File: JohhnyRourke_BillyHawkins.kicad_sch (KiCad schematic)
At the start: 12 parts, among them J1 Power In, J2 Motor Out, U2 DRV8873HPWPRQ1

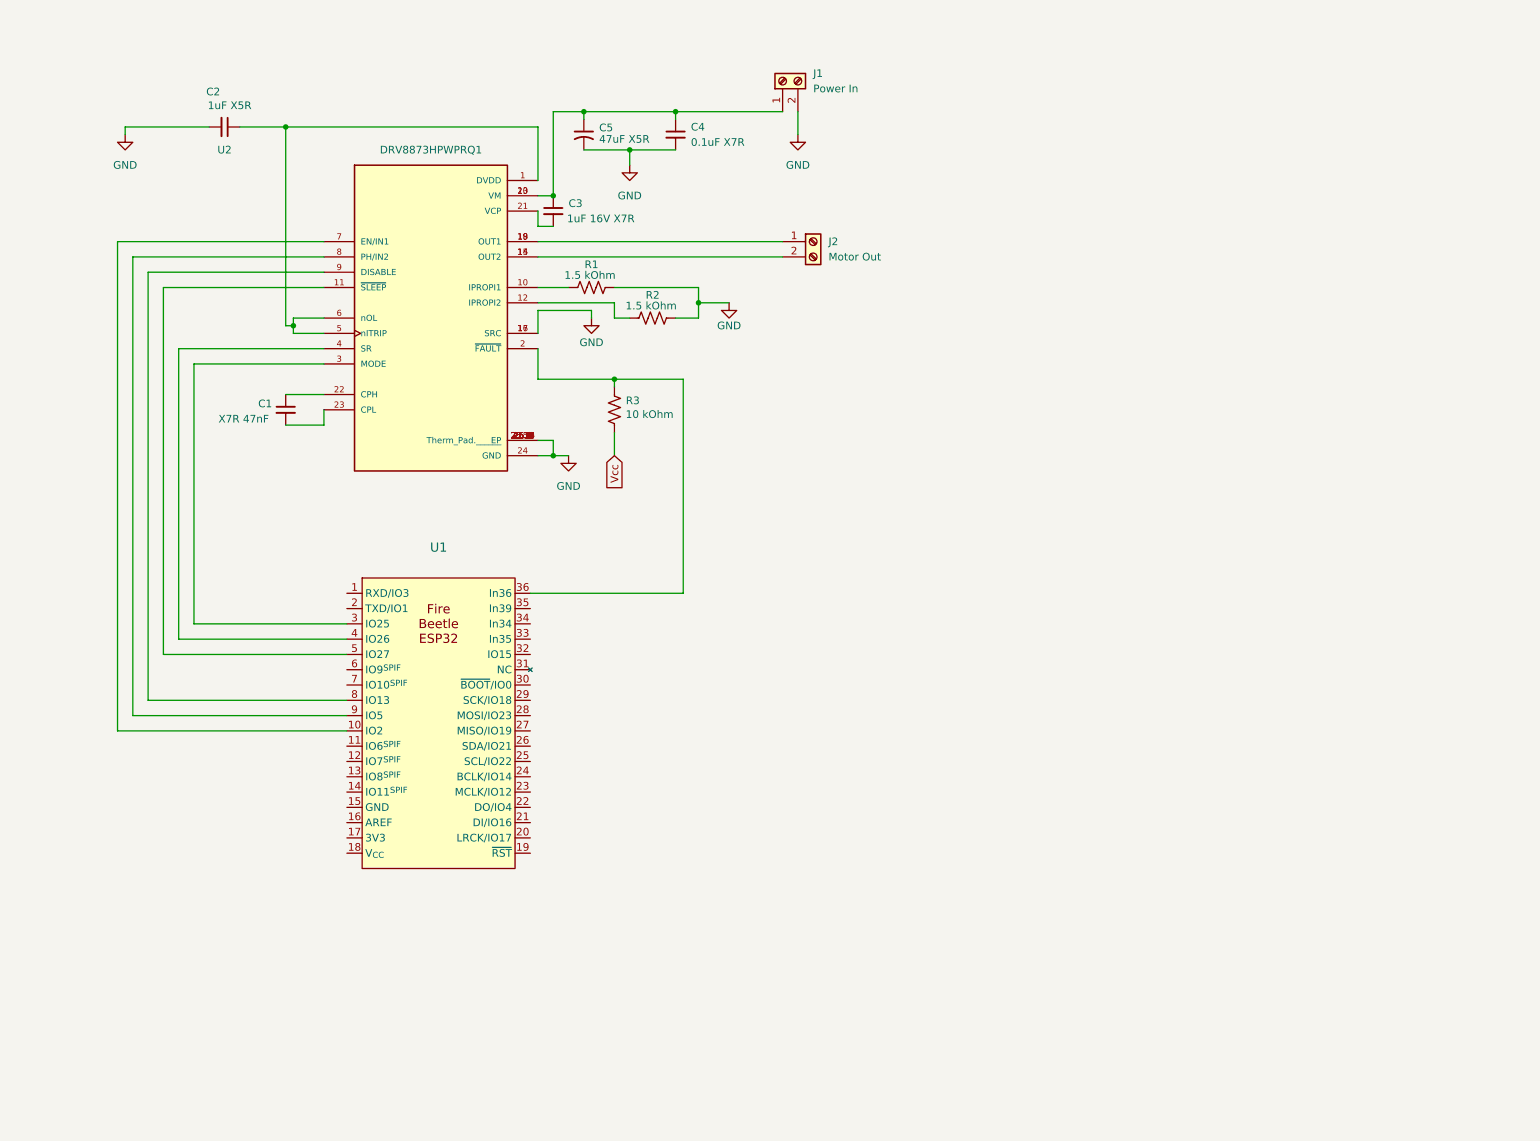
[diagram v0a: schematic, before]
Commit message: Add files via upload
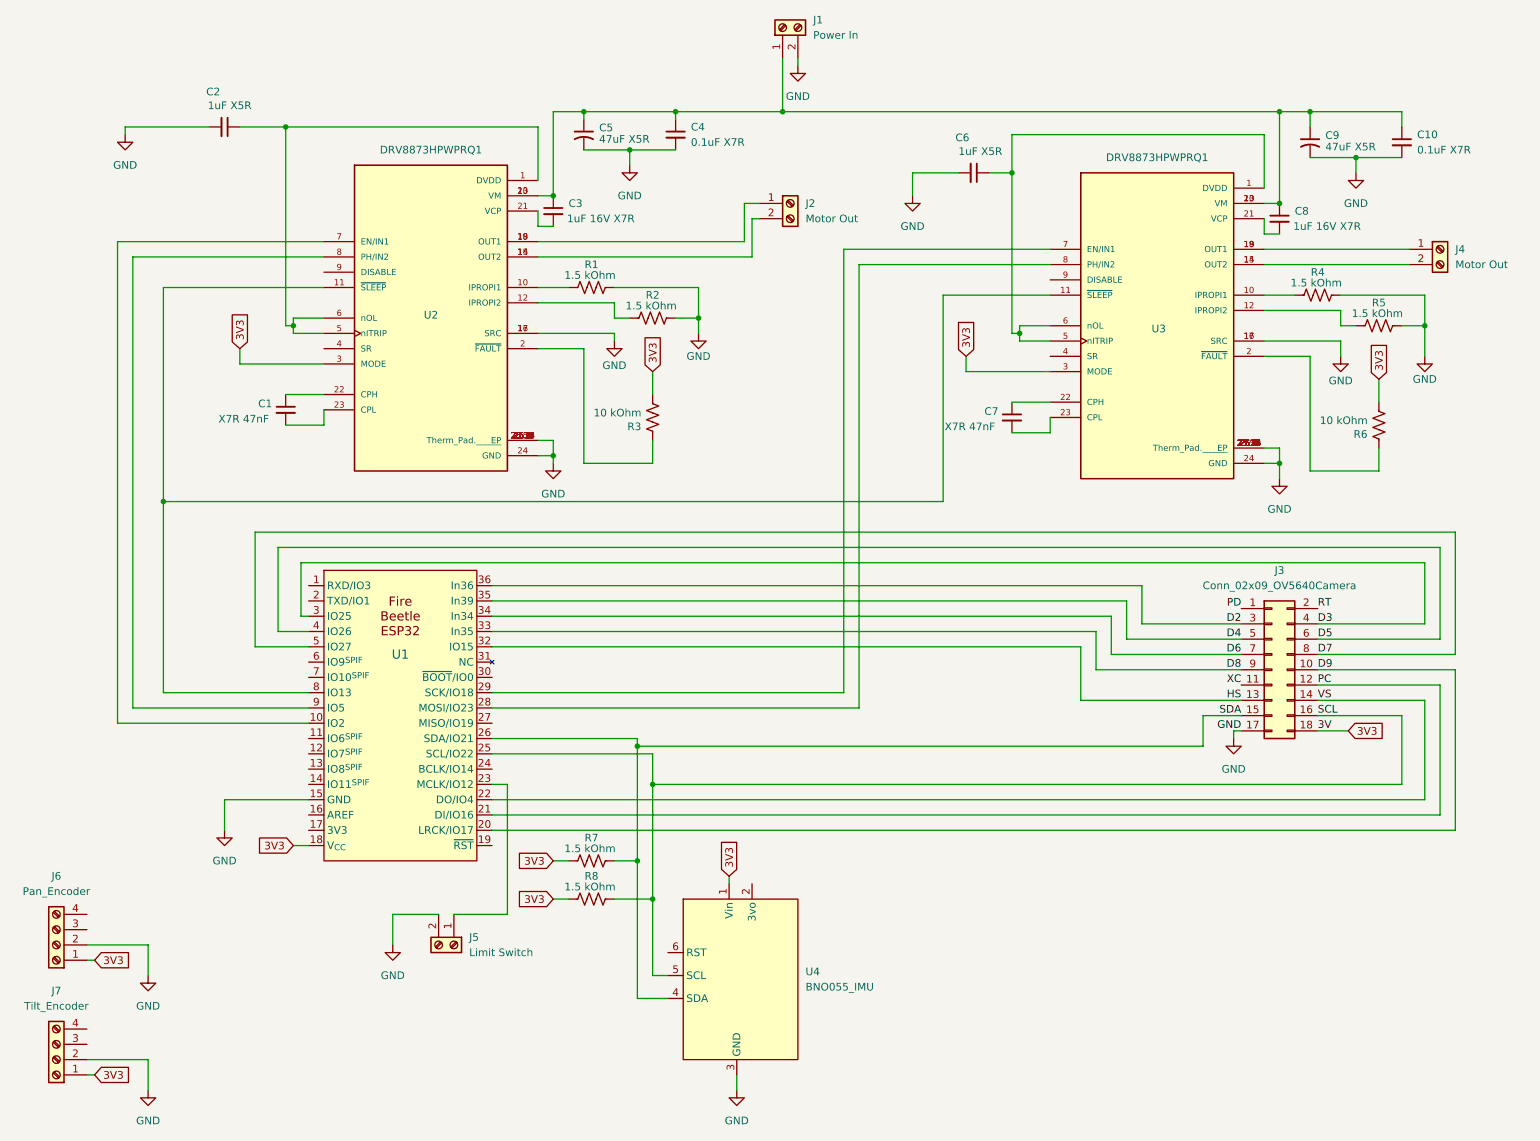
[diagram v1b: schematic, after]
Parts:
- added C10: 0.1uF X7R, Capacitor_SMD:C_0805_2012Metric_Pad1.18x1.45mm_HandSolder, symbol Device:C_Small
- added C6: 1uF X5R, Capacitor_SMD:C_0805_2012Metric_Pad1.18x1.45mm_HandSolder, symbol Device:C_Small
- added C7: X7R 47nF, Capacitor_SMD:C_0805_2012Metric_Pad1.18x1.45mm_HandSolder, symbol Device:C_Small
- added C8: 1uF 16V X7R, Capacitor_SMD:C_0805_2012Metric_Pad1.18x1.45mm_HandSolder, symbol Device:C_Small
- added C9: 47uF X5R, Capacitor_SMD:C_1206_3216Metric_Pad1.33x1.80mm_HandSolder, symbol Device:C_Small_US
- added J3: Conn_02x09_OV5640Camera, symbol Connector_Generic:Conn_02x09_Odd_Even
- added J4: Motor Out, TerminalBlock_Phoenix:TerminalBlock_Phoenix_MKDS-1,5-2_1x02_P5.00mm_Horizontal, symbol Connector:Screw_Terminal_01x02
- added J5: Limit Switch, symbol Connector:Screw_Terminal_01x02
- added J6: Pan_Encoder, symbol Connector:Screw_Terminal_01x04
- added J7: Tilt_Encoder, symbol Connector:Screw_Terminal_01x04
- added R4, R5, R7, R8: 1.5 kOhm, Resistor_SMD:R_0805_2012Metric_Pad1.20x1.40mm_HandSolder, symbol Device:R_US
- added R6: 10 kOhm, Resistor_SMD:R_0805_2012Metric_Pad1.20x1.40mm_HandSolder, symbol Device:R_US
- added U3: DRV8873HPWPRQ1, DRV8873SPWPRQ1:IC_DRV8873SPWPRQ1, symbol DRV8873SPWPRQ1:DRV8873SPWPRQ1
- added U4: BNO055_IMU, symbol BNO055:BNO055
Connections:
- net Vcc is gone; now on net 3V3: R3.2
- net GND: now also U1.15 (GND), C10.2, C6.2, C9.2, J3.17 (Pin_17), J5.2 (Pin_2), J6.2 (Pin_2), J7.2 (Pin_2), R4.2, R5.2, U3.16 (SRC), U3.17 (SRC), U3.24 (GND), U3.25 (Therm_Pad.______), U3.25.1 (EP), U3.25.10 (EP), U3.25.11 (EP), U3.25.12 (EP), U3.25.13 (EP), U3.25.14 (EP), U3.25.15 (EP), U3.25.16 (EP), U3.25.17 (EP), U3.25.18 (EP), U3.25.2 (EP), U3.25.3 (EP), U3.25.4 (EP), U3.25.5 (EP), U3.25.6 (EP), U3.25.7 (EP), U3.25.8 (EP), U3.25.9 (EP), U4.3 (GND)
- net at U2.11 (~{SLEEP}): now also U1.8 (IO13), U3.11 (~{SLEEP}); no longer U1.5 (IO27)
- net at C3.1, C4.1, C5.1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: now also C10.1, C8.1, C9.1, U3.13 (VM), U3.20 (VM)
- net at R3.1, U2.2 (~{FAULT}): no longer U1.36 (In36)
- net 3V3: now reaches U2.3 (MODE)
- net 3V3: now also U1.18 (V_{CC}), J3.18 (Pin_18), J6.1 (Pin_1), J7.1 (Pin_1), R6.2, R7.1, R8.1, U3.3 (MODE), U4.1 (Vin); no longer U1.3 (IO25)
- net at U2.4 (SR): no longer U1.4 (IO26)
- net at U2.9 (DISABLE): no longer U1.8 (IO13)
- net D9: now reaches U1.20 (LRCK/IO17)
- net D9: now also J3.10 (Pin_10)
- net PC: now reaches U1.21 (DI/IO16)
- net PC: now also J3.12 (Pin_12)
- net VS: now reaches U1.22 (DO/IO4)
- net VS: now also J3.14 (Pin_14)
- net at U1.23 (MCLK/IO12): now also J5.1 (Pin_1)
- net SCL: now reaches U1.25 (SCL/IO22)
- net SCL: now also J3.16 (Pin_16), R8.2, U4.5 (SCL)
- net SDA: now reaches U1.26 (SDA/IO21)
- net SDA: now also J3.15 (Pin_15), R7.2, U4.4 (SDA)
- net at U1.28 (MOSI/IO23): now also U3.8 (PH/IN2)
- net at U1.29 (SCK/IO18): now also U3.7 (EN/IN1)
- net HS: now reaches U1.32 (IO15)
- net HS: now also J3.13 (Pin_13)
- net D8: now reaches U1.33 (In35)
- net D8: now also J3.9 (Pin_9)
- net D6: now reaches U1.34 (In34)
- net D6: now also J3.7 (Pin_7)
- net D4: now reaches U1.35 (In39)
- net D4: now also J3.5 (Pin_5)
- new net: J4.1 (Pin_1), U3.18 (OUT1), U3.19 (OUT1)
- new net: J4.2 (Pin_2), U3.14 (OUT2), U3.15 (OUT2)
- new net: C6.1, U3.1 (DVDD), U3.5 (nITRIP), U3.6 (nOL)
- new net: R4.1, U3.10 (IPROPI1)
- new net: R5.1, U3.12 (IPROPI2)
- new net: R6.1, U3.2 (~{FAULT})
- new net: C8.2, U3.21 (VCP)
- new net: C7.1, U3.22 (CPH)
- new net: C7.2, U3.23 (CPL)
- new net D2: J3.3 (Pin_3), U1.36 (In36)
- new net D3: J3.4 (Pin_4), U1.3 (IO25)
- new net D5: J3.6 (Pin_6), U1.4 (IO26)
- new net D7: J3.8 (Pin_8), U1.5 (IO27)
- new net PD: J3.1 (Pin_1)
- new net RT: J3.2 (Pin_2)
- new net XC: J3.11 (Pin_11)
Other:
- moved on the sheet: J1, J2, R3, U1
